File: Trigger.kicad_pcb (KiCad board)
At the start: 2 copper layers, 20 x 40 mm, 11 parts, among them P1 CONN_01X03, U1 MCP6002

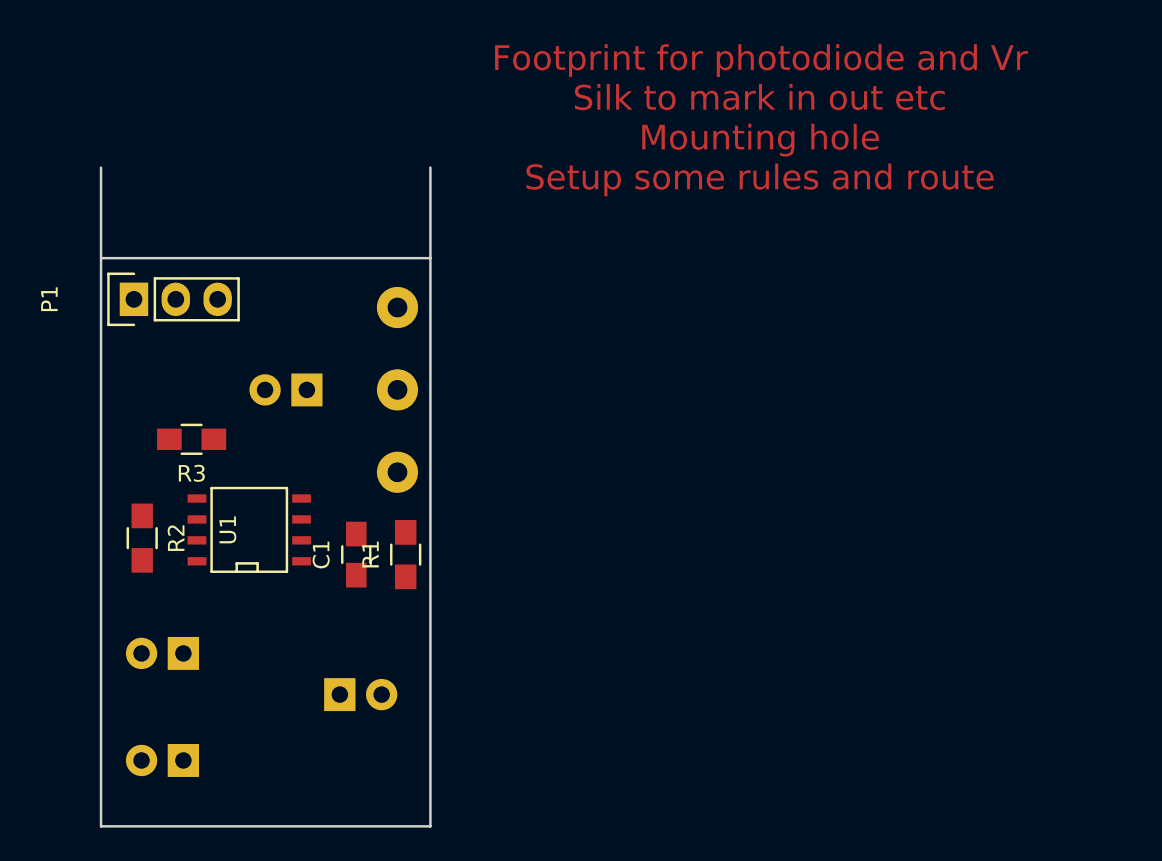
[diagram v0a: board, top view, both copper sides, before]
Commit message: As submitted
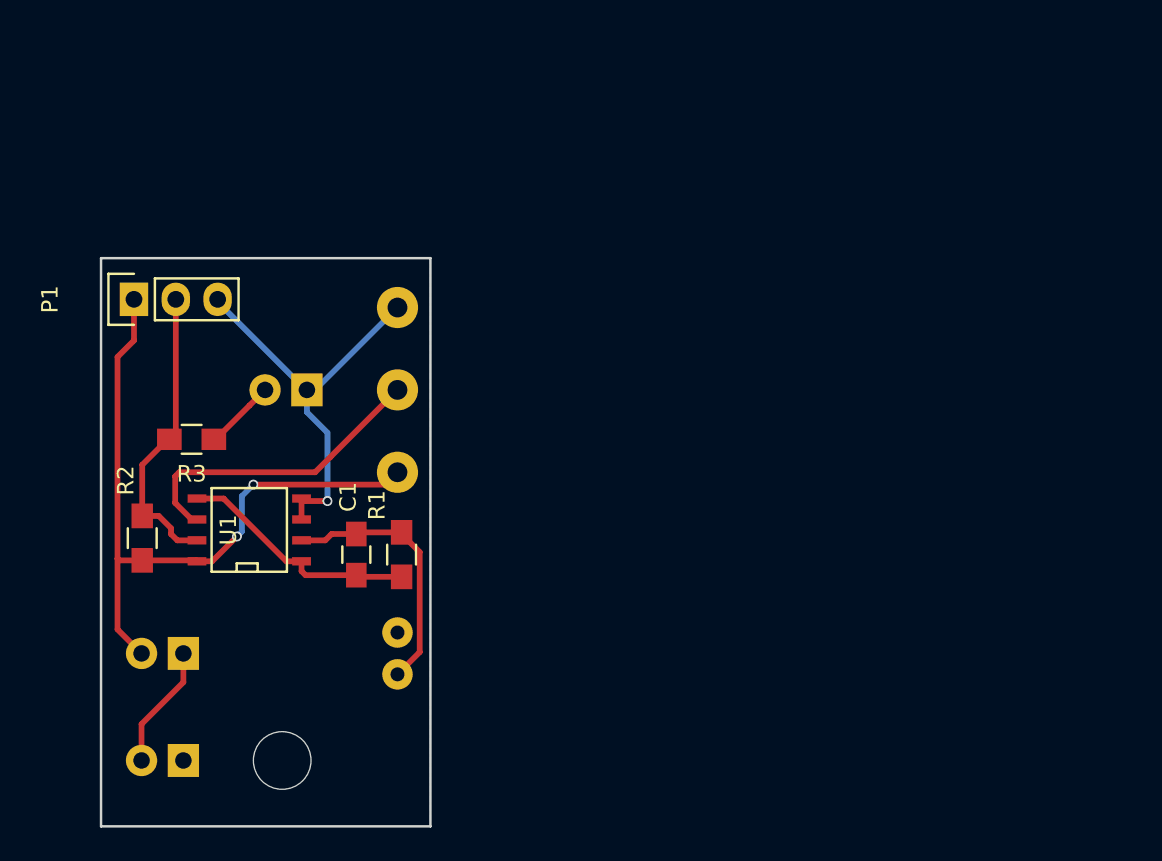
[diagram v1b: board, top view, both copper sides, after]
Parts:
- added H1: MountHole, Mounting_Holes:MountingHole_3.5mm, F.Cu at (95.0, 130.0)
- D3: footprint LEDs:LED-5MM -> SMD_Mine:PhotoDiode
- RV2: footprint Potentiometers:Potentiometer_WirePads_largePads -> SMD_Mine:Potentiometer_WirePads_largePads
- moved D3 4.30 mm to (102.0, 123.5)
- moved R1 0.25 mm to (102.2, 117.5)
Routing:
- net +3V3: track 0.00 -> 43.1 mm, vias 0 -> 2
- net GND: track 0.00 -> 25.5 mm, vias 0 -> 1
- net Net-(RV2-Pad2): track 0.00 -> 19.0 mm
- net Net-(P1-Pad2): track 0.00 -> 18.2 mm
- net Net-(C1-Pad2): track 0.00 -> 15.9 mm
- net Net-(C1-Pad1): track 0.00 -> 14.7 mm
- net Net-(D1-Pad1): track 0.00 -> 7.55 mm
- net Net-(D4-Pad2): track 0.00 -> 4.35 mm
- added copper zone on B.Cu, net GND
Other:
- board size 20 x 40 mm -> 20 x 34.5 mm
- net class Default: clearance 0.2 -> 0.25; trace_width 0.25 -> 0.35
- rule trace_clearance: 0.2 -> 0.25
- board text added: "+3v"
- board text added: "G"
- board text added: "IR Trigger"
- board text added: "Tr"
- board text removed: "Footprint for photodiode and Vr Silk to mark in out etc Mounting hole Setup some rules and route"
